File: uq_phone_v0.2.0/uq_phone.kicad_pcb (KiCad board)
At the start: 6 copper layers, 130.1 x 108 mm, 201 parts, among them J1 PJ-242C, J10 513382474, J11 513382474, J2 124018312112A, J3 BM03B-ACHSS-GAN-TF_LF__SN_, J4 20279-001E-03, J5 20279-001E-03, J6 Conn_ARM_SWD_TagConnect_TC2030, J7 559092474, J8 MCS-302S-C1, J9 559092474, M1 C08-00A, Q1 MMBT3904LP-7, Q2 MMBT3904LP-7, Q3 S8050, SW1 SKTAAAE010, SW10 SKTAAAE010, SW11 SKTAAAE010, SW12 SKTAAAE010, SW13 SKTAAAE010, SW14 SKTAAAE010, SW15 SKTAAAE010, SW16 SKSCLCE010, SW17 SKTAAAE010, SW18 SKTAAAE010, SW19 SKTAAAE010, SW2 SKTAAAE010, SW20 SKTAAAE010, SW21 SKTAAAE010, SW22 SKSCLCE010, SW23 SKTAAAE010, SW24 SKTAAAE010, SW25 SKTAAAE010, SW26 SKTAAAE010, SW27 SKTAAAE010, SW28 SKTAAAE010, SW29 SKTAAAE010, SW3 SKTAAAE010, SW30 SKTAAAE010, SW31 SKTAAAE010, SW32 SKTAAAE010, SW33 SKTAAAE010, SW34 SKTAAAE010, SW35 SKTAAAE010, SW36 SKTAAAE010, SW37 SKTAAAE010, SW38 SKTAAAE010, SW39 SKTAAAE010, SW4 SKTAAAE010, SW40 SKTAAAE010, SW41 SKTAAAE010, SW5 SKTAAAE010, SW6 SKSCLCE010, SW7 SKTAAAE010, SW8 SKTAAAE010, SW9 SKTAAAE010, U1 TPS62162DSGR, U10 TPD8F003DQDR, U11 LSM6DSVTR, U12 DRV2603RUNR, U13 TS3A5018RSVR, U14 NAU88C22YG, U15 TPS22964CYZPR, U16 TXB0108YZPR2, U2 MCP73871-2CCI_ML, U3 BQ27441DRZR-G1A, U4 WP SNAP-IN BASE_6000636, U5 TCA9509MRVHR, U6 STM32H733VGHx, U7 TXB0108YZPR2, U8 TPD3F303DQDR

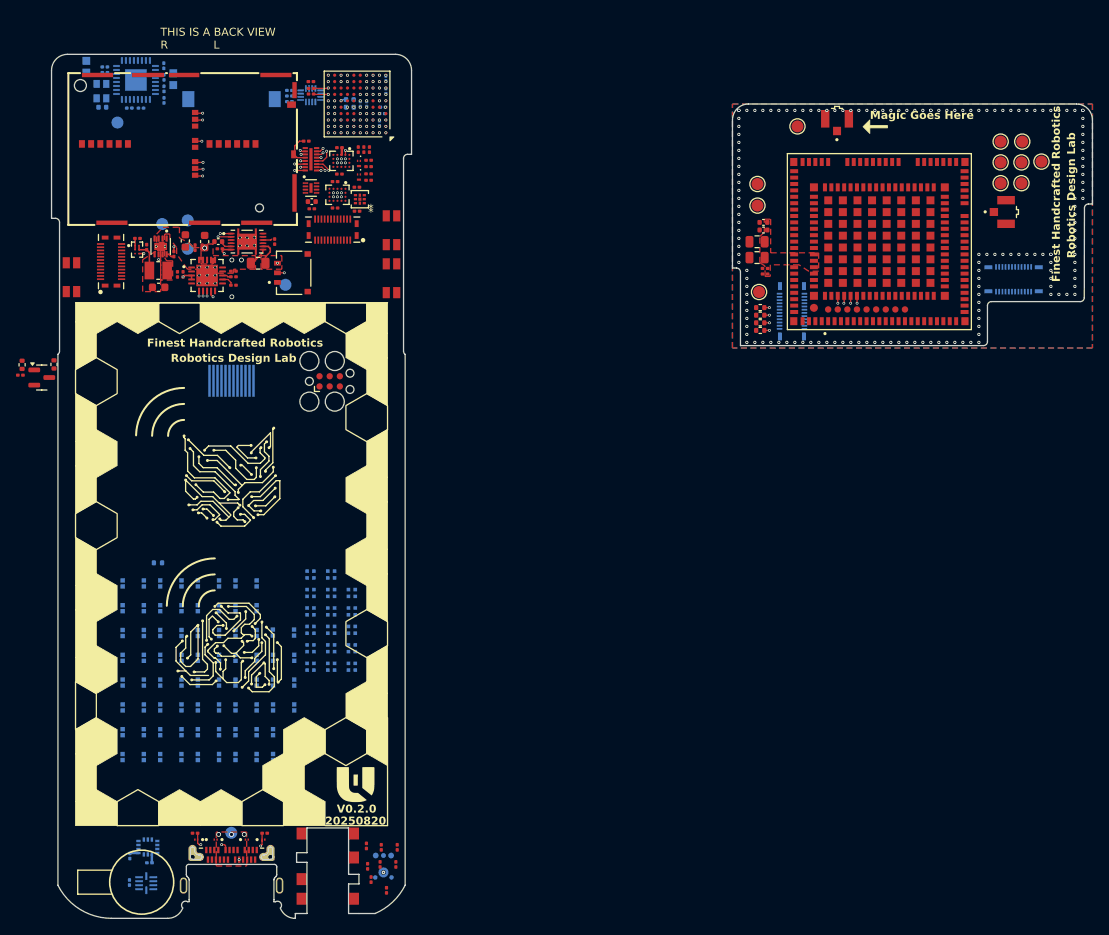
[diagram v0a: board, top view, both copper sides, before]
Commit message: Several Hours of Routing
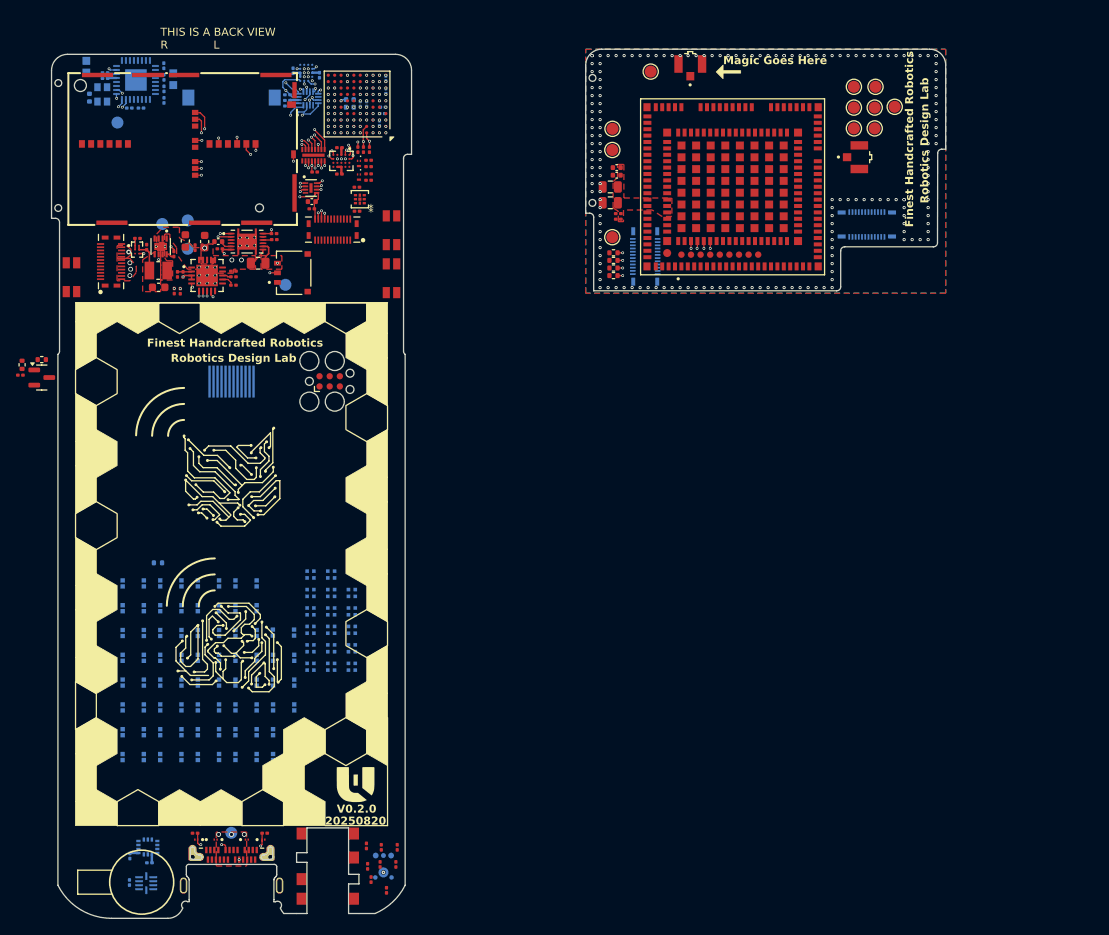
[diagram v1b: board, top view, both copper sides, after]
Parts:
- added ?: , , F.Cu at (85.9, 39.5)
- added ?: , , F.Cu at (85.9, 23.8)
- added REF**: MountingHole, custom_footprints:Mounting, F.Cu at (19.1, 24.5)
- added REF**: MountingHole, custom_footprints:Mounting, F.Cu at (19.1, 40.1)
- C23, C24, U7: moved to B.Cu
- R27: value 10R -> 5R
- moved R23 30.2 mm to (34.4, 50.5), turned to -90 degrees
- moved R24 30.0 mm to (33.6, 50.5), turned to -90 degrees
- moved J10 19.6 mm to (120.2, 42.2)
- moved C10 19.6 mm to (89.1, 41.5)
- moved C11 19.6 mm to (89.1, 40.8)
- moved C12 19.6 mm to (88.1, 39.5)
- moved C13 19.6 mm to (88.1, 37.5)
- moved C8 19.6 mm to (88.9, 36.0)
- moved C9 19.6 mm to (88.9, 35.0)
- moved J11 19.6 mm to (92.5, 46.2)
- moved J4 19.6 mm to (98.1, 22.1)
- moved R12 19.6 mm to (88.5, 47.6)
- moved R13 19.6 mm to (88.5, 45.7)
- moved R14 19.6 mm to (88.5, 48.5)
- moved R15 19.6 mm to (88.5, 46.6)
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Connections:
- J11 pad 1: VBAT -> GND
- J11 pad 10: +1.8V -> GND
- J11 pad 11: +1.8V -> GND
- J11 pad 12: +1.8V -> GND
- J11 pad 13: GND -> VBAT
- J11 pad 14: GND -> VBAT
- J11 pad 15: GND -> VBAT
- J11 pad 16: GND -> VBAT
- J11 pad 17: GND -> VBAT
- J11 pad 18: GND -> VBAT
- J11 pad 19: GND -> VBAT
- J11 pad 2: VBAT -> GND
- J11 pad 20: GND -> +1.8V
- J11 pad 21: GND -> +1.8V
- J11 pad 22: GND -> +1.8V
- J11 pad 23: GND -> +1.8V
- J11 pad 3: VBAT -> GND
- J11 pad 4: VBAT -> GND
- J11 pad 5: VBAT -> GND
- J11 pad 6: VBAT -> GND
- J11 pad 7: VBAT -> GND
- J11 pad 8: VBAT -> GND
- J11 pad 9: +1.8V -> GND
- J7 pad 1: VBAT -> GND
- J7 pad 10: +1.8V -> GND
- J7 pad 11: +1.8V -> GND
- J7 pad 12: +1.8V -> GND
- J7 pad 13: GND -> VBAT
- J7 pad 14: GND -> VBAT
- J7 pad 15: GND -> VBAT
- J7 pad 16: GND -> VBAT
- J7 pad 17: GND -> VBAT
- J7 pad 18: GND -> VBAT
- J7 pad 19: GND -> VBAT
- J7 pad 2: VBAT -> GND
- J7 pad 20: GND -> +1.8V
- J7 pad 21: GND -> +1.8V
- J7 pad 22: GND -> +1.8V
- J7 pad 23: GND -> +1.8V
- J7 pad 3: VBAT -> GND
- J7 pad 4: VBAT -> GND
- J7 pad 5: VBAT -> GND
- J7 pad 6: VBAT -> GND
- J7 pad 7: VBAT -> GND
- J7 pad 8: VBAT -> GND
- J7 pad 9: +1.8V -> GND
- J9 pad 21: unconnected-(J9-Pad21) -> SIM_RST
- J9 pad 22: unconnected-(J9-Pad22) -> SIM_CLK
- J9 pad 23: unconnected-(J9-Pad23) -> SIM_DATA
- J9 pad 24: unconnected-(J9-Pad24) -> SIM_VDD
- U16 pad A1: MCU_DCD -> MCU_DTR
- U16 pad A2: MCU_DSR -> MCU_DCD
- U16 pad A3: MOB_DSR -> MOB_DCD
- U16 pad A4: MOB_DCD -> MOB_DTR
- U16 pad B1: MCU_RXD -> MCU_DSR
- U16 pad B2: MCU_DTR -> MCU_TXD
- U16 pad B3: MOB_DTR -> MOB_TXD
- U16 pad B4: MOB_RXD -> MOB_DSR
- U16 pad C2: MCU_TXD -> MCU_RTS
- U16 pad C3: MOB_TXD -> MOB_RTS
- U16 pad D2: MCU_RTS -> MCU_CTS
- U16 pad D3: MOB_RTS -> MOB_CTS
- U16 pad E1: MCU_CTS -> MCU_RXD
- U16 pad E4: MOB_CTS -> MOB_RXD
- U6 pad C7: unconnected-(U6-PD3-PadC7) -> MCU_DCD
- U6 pad D8: unconnected-(U6-PD0-PadD8) -> MCU_DTR
- U6 pad G10: MCP_STAT1 -> MCP_PG
- U6 pad G9: unconnected-(U6-PD11-PadG9) -> FUEL_GPO
- U6 pad H10: MCP_STAT2 -> MCP_STAT1
- U6 pad H9: unconnected-(U6-PD10-PadH9) -> MCP_STAT2
- U6 pad J10: MCU_DTR -> unconnected-(U6-PD13-PadJ10)
- U6 pad J8: MCP_PG -> unconnected-(U6-PB13-PadJ8)
- U6 pad K10: MCU_DCD -> unconnected-(U6-PD12-PadK10)
- U6 pad K8: FUEL_GPO -> unconnected-(U6-PB12-PadK8)
- U7 pad B1: HP_DET_MCU -> MCU_AUD_OUT_L_H
- U7 pad B2: MOB_WAKE_H -> MCU_AUD_BCLK_H
- U7 pad B3: MOB_WAKE_L -> MCU_AUD_BCLK_L
- U7 pad B4: HP_DET -> MCU_AUD_OUT_L
- U7 pad D2: MCU_AUD_BCLK_H -> MOB_WAKE_H
- U7 pad D3: MCU_AUD_BCLK_L -> MOB_WAKE_L
- U7 pad E2: MCU_AUD_OUT_L_H -> HP_DET_MCU
- U7 pad E3: MCU_AUD_OUT_L -> HP_DET
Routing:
- net FUEL_GPO: track 0.00 -> 43.7 mm, vias 1 -> 2
- net MCP_STAT1: track 2.48 -> 46.1 mm, vias 2 -> 3
- net MCP_STAT2: track 2.48 -> 44.9 mm, vias 2 -> 3
- net MCP_PG: track 0.63 -> 42.2 mm
- net AUD_OUT: track 0.00 -> 29.8 mm, vias 0 -> 2
- net AUD_IN: track 0.00 -> 28.5 mm, vias 0 -> 2
- net AUD_BCLK: track 0.00 -> 28.3 mm, vias 0 -> 2
- net HP_DET: track 0.00 -> 26.8 mm, vias 0 -> 2
- net AUD_SYNC: track 0.00 -> 25.9 mm, vias 0 -> 2
- net SIM_VDD: track 0.00 -> 20.1 mm, vias 0 -> 2
- net Net-(J8B-SIM_1_RST): track 0.00 -> 12.5 mm, vias 0 -> 2
- net MCU_AUD_BCLK_H: track 0.00 -> 11.6 mm
- net MCU_AUD_SYNC_H: track 0.00 -> 11.4 mm
- net BAT_THERM: track 0.85 -> 11.9 mm, vias 1 -> 2
- net Net-(J8B-SIM_1_DATA): track 0.00 -> 10.6 mm, vias 0 -> 2
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- added copper zone on F.Cu, net +1.8V
- added copper zone on In2.Cu, net VBAT
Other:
- board size 130.1 x 108 mm -> 111.8 x 108.6 mm
